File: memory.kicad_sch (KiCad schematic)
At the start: 4 parts

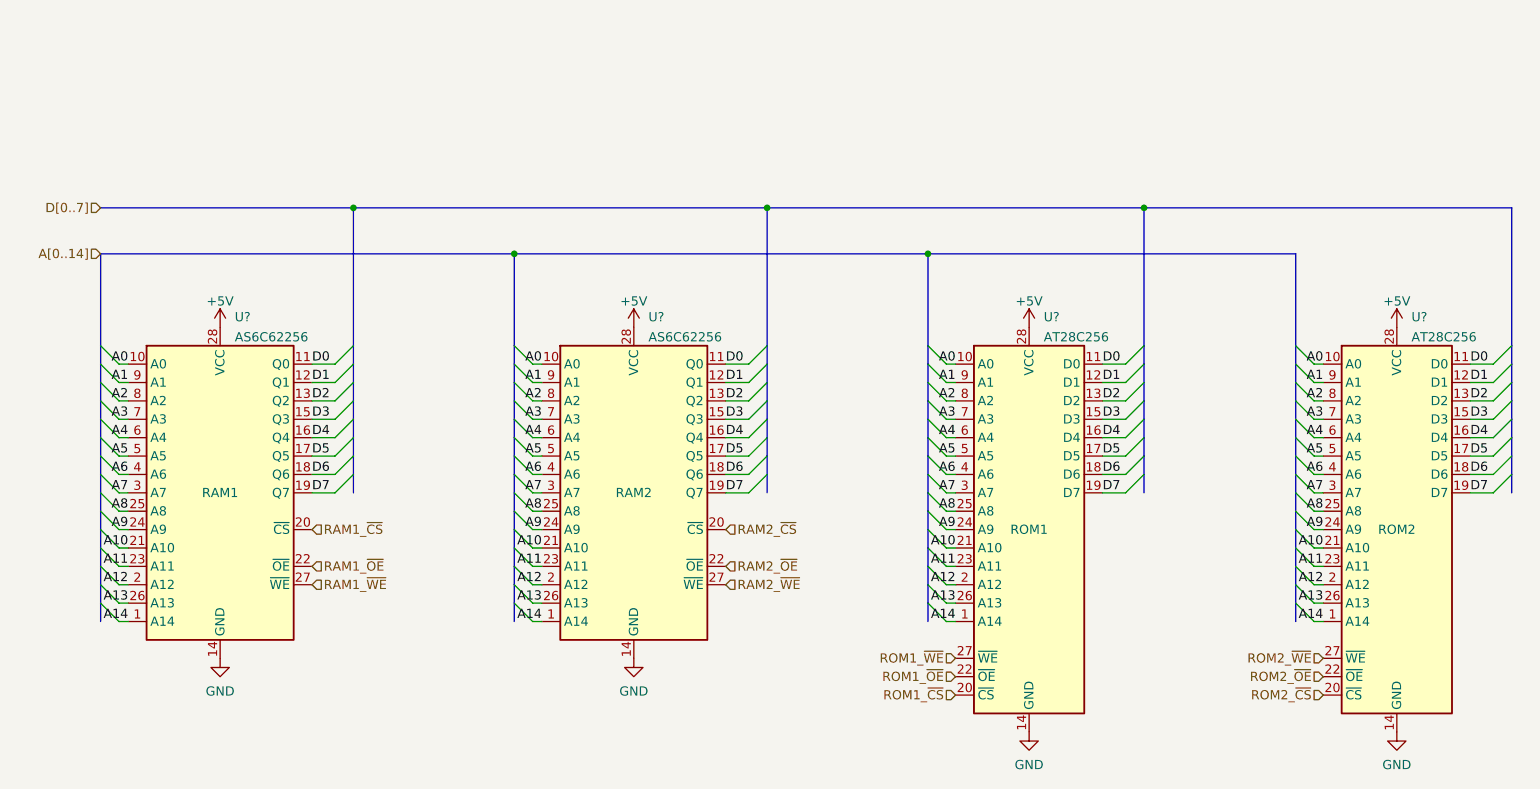
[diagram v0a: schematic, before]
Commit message: Final PCB Layout
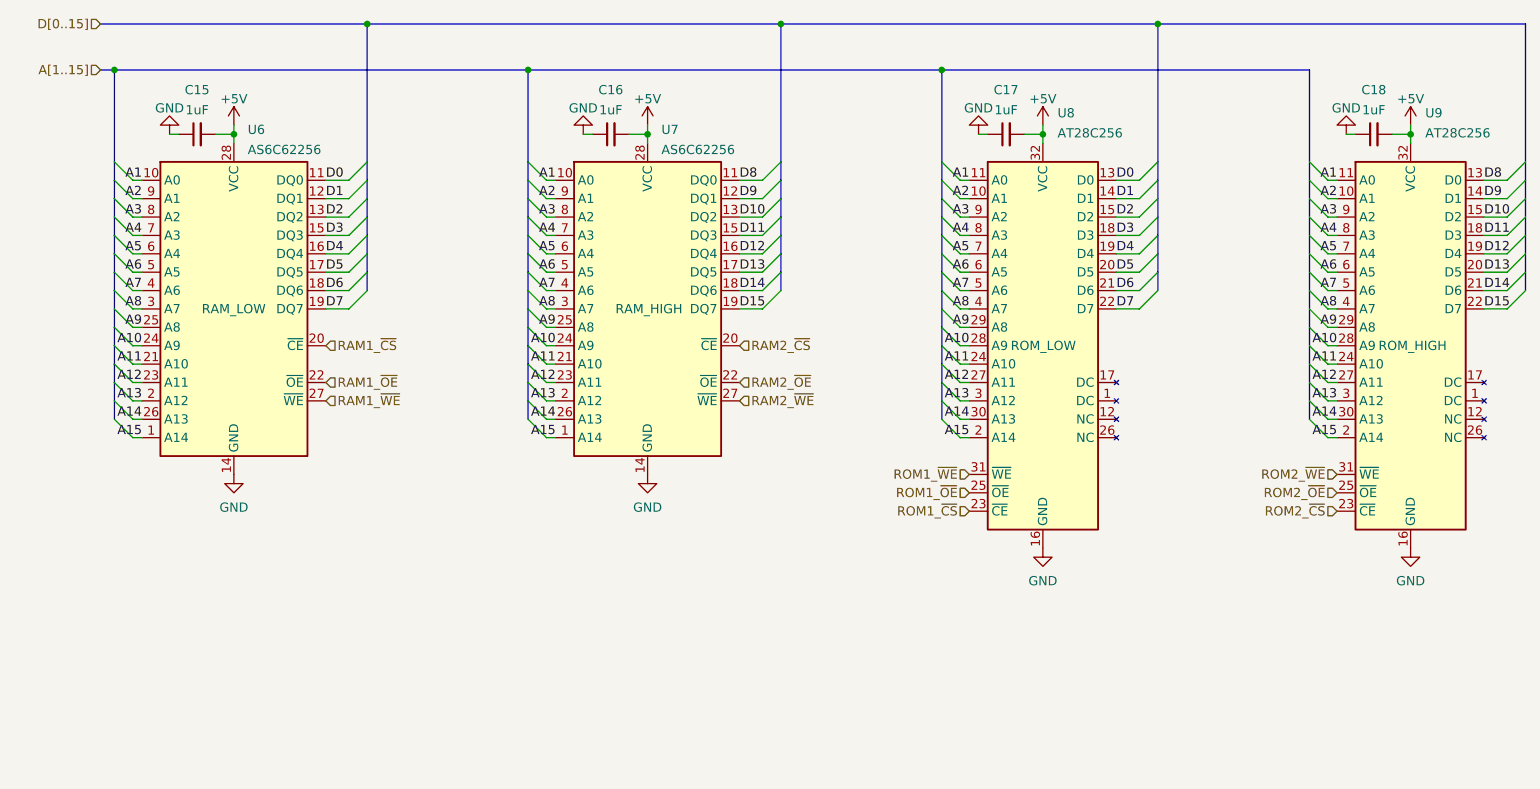
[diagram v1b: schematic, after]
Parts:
- added C15, C16, C17, C18: 1uF, Capacitor_SMD:C_0805_2012Metric_Pad1.18x1.45mm_HandSolder, symbol Device:C_Small
- U6: renamed from U?; footprint Package_DIP:DIP-28_W15.24mm -> Package_DIP:DIP-28_W15.24mm_Socket_LongPads; symbol Memory_RAM:KM62256CLP -> MCD_Symbols:AS6C62256; Name RAM1 -> RAM_LOW
- U7: renamed from U?; footprint Package_DIP:DIP-28_W15.24mm -> Package_DIP:DIP-28_W15.24mm_Socket_LongPads; symbol Memory_RAM:KM62256CLP -> MCD_Symbols:AS6C62256; Name RAM2 -> RAM_HIGH
- U8: renamed from U?; footprint Package_LCC:PLCC-32_11.4x14.0mm_P1.27mm -> Package_LCC:PLCC-32_THT-Socket; symbol Memory_EEPROM:28C256 -> MCD_Symbols:AT28C256; Name ROM1 -> ROM_LOW
- U9: renamed from U?; footprint Package_LCC:PLCC-32_11.4x14.0mm_P1.27mm -> Package_LCC:PLCC-32_THT-Socket; symbol Memory_EEPROM:28C256 -> MCD_Symbols:AT28C256; Name ROM2 -> ROM_HIGH
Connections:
- net +5V: now also U8.32 (VCC), U9.32 (VCC), C15.2, C16.2, C17.2, C18.2; no longer U8.28 (VCC), U9.28 (VCC)
- net A1: now also U6.10 (A0), U7.10 (A0), U8.11 (A0), U9.11 (A0); no longer U6.9 (A1), U7.9 (A1), U8.9 (A1), U9.9 (A1)
- net A10: now also U6.24 (A9), U7.24 (A9), U8.28 (A9), U9.28 (A9); no longer U6.21 (A10), U7.21 (A10), U8.21 (A10), U9.21 (A10)
- net A11: now also U6.21 (A10), U7.21 (A10), U8.24 (A10), U9.24 (A10); no longer U6.23 (A11), U7.23 (A11), U8.23 (A11), U9.23 (A11)
- net A12: now also U6.23 (A11), U7.23 (A11), U8.27 (A11), U9.27 (A11); no longer U6.2 (A12), U7.2 (A12), U8.2 (A12), U9.2 (A12)
- net A13: now also U6.2 (A12), U7.2 (A12), U8.3 (A12), U9.3 (A12); no longer U6.26 (A13), U7.26 (A13), U8.26 (A13), U9.26 (A13)
- net A14: now also U6.26 (A13), U7.26 (A13), U8.30 (A13), U9.30 (A13); no longer U6.1 (A14), U7.1 (A14), U8.1 (A14), U9.1 (A14)
- net A2: now also U6.9 (A1), U7.9 (A1), U8.10 (A1), U9.10 (A1); no longer U6.8 (A2), U7.8 (A2), U8.8 (A2), U9.8 (A2)
- net A3: now also U6.8 (A2), U7.8 (A2), U8.9 (A2), U9.9 (A2); no longer U6.7 (A3), U7.7 (A3), U8.7 (A3), U9.7 (A3)
- net A4: now also U6.7 (A3), U7.7 (A3), U8.8 (A3), U9.8 (A3); no longer U6.6 (A4), U7.6 (A4), U8.6 (A4), U9.6 (A4)
- net A5: now also U6.6 (A4), U7.6 (A4), U8.7 (A4), U9.7 (A4); no longer U6.5 (A5), U7.5 (A5), U8.5 (A5), U9.5 (A5)
- net A6: now also U6.5 (A5), U7.5 (A5), U8.6 (A5), U9.6 (A5); no longer U6.4 (A6), U7.4 (A6), U8.4 (A6), U9.4 (A6)
- net A7: now also U6.4 (A6), U7.4 (A6), U8.5 (A6), U9.5 (A6); no longer U6.3 (A7), U7.3 (A7), U8.3 (A7), U9.3 (A7)
- net A8: now also U6.3 (A7), U7.3 (A7), U8.4 (A7), U9.4 (A7); no longer U6.25 (A8), U7.25 (A8), U8.25 (A8), U9.25 (A8)
- net A9: now also U6.25 (A8), U7.25 (A8), U8.29 (A8), U9.29 (A8); no longer U6.24 (A9), U7.24 (A9), U8.24 (A9), U9.24 (A9)
- net D0: now also U8.13 (D0); no longer U7.11 (Q0), U8.11 (D0), U9.11 (D0)
- net D1: now also U8.14 (D1); no longer U7.12 (Q1), U8.12 (D1), U9.12 (D1)
- net D2: now also U8.15 (D2); no longer U7.13 (Q2), U8.13 (D2), U9.13 (D2)
- net D3: now also U8.18 (D3); no longer U7.15 (Q3), U8.15 (D3), U9.15 (D3)
- net D4: now also U8.19 (D4); no longer U7.16 (Q4), U8.16 (D4), U9.16 (D4)
- net D5: now also U8.20 (D5); no longer U7.17 (Q5), U8.17 (D5), U9.17 (D5)
- net D6: now also U8.21 (D6); no longer U7.18 (Q6), U8.18 (D6), U9.18 (D6)
- net D7: now also U8.22 (D7); no longer U7.19 (Q7), U8.19 (D7), U9.19 (D7)
- net GND: now also U8.16 (GND), U9.16 (GND), C15.1, C16.1, C17.1, C18.1; no longer U8.14 (GND), U9.14 (GND)
- net ROM1_~{CS}: now also U8.23 (~{CE}); no longer U8.20 (~{CS})
- net ROM1_~{OE}: now also U8.25 (~{OE}); no longer U8.22 (~{OE})
- net ROM1_~{WE}: now also U8.31 (~{WE}); no longer U8.27 (~{WE})
- net ROM2_~{CS}: now also U9.23 (~{CE}); no longer U9.20 (~{CS})
- net ROM2_~{OE}: now also U9.25 (~{OE}); no longer U9.22 (~{OE})
- net ROM2_~{WE}: now also U9.31 (~{WE}); no longer U9.27 (~{WE})
- removed net A0: U6.10 (A0), U7.10 (A0), U8.10 (A0), U9.10 (A0)
- new net A15: U6.1 (A14), U7.1 (A14), U8.2 (A14), U9.2 (A14)
- new net D10: U7.13 (DQ2), U9.15 (D2)
- new net D11: U7.15 (DQ3), U9.18 (D3)
- new net D12: U7.16 (DQ4), U9.19 (D4)
- new net D13: U7.17 (DQ5), U9.20 (D5)
- new net D14: U7.18 (DQ6), U9.21 (D6)
- new net D15: U7.19 (DQ7), U9.22 (D7)
- new net D8: U7.11 (DQ0), U9.13 (D0)
- new net D9: U7.12 (DQ1), U9.14 (D1)
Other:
- company: (none) -> Jackson Miller
- title: (none) -> Memory Connections
- moved on the sheet: U6, U7
